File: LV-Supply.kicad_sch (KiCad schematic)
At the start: 20 parts, among them U11 LMR16006XDDCR

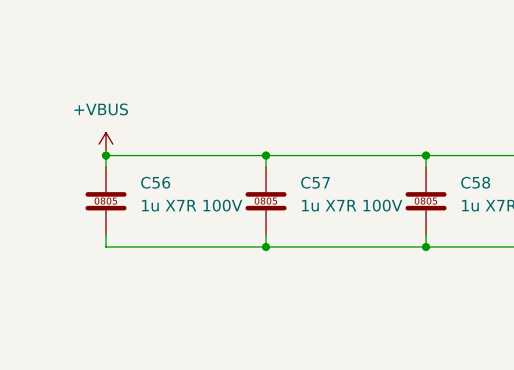
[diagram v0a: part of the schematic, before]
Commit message: Finished layout
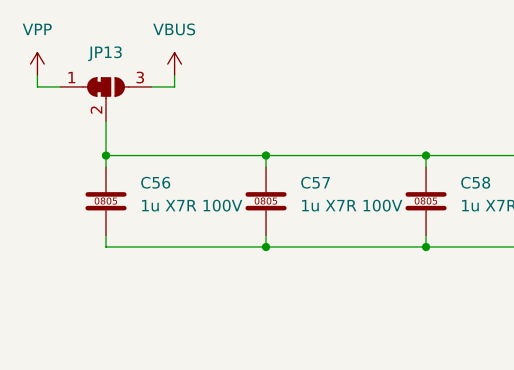
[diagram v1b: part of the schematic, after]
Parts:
- added JP13: SolderJumper_3_Bridged12, Jumper:SolderJumper-3_P1.3mm_Bridged12_RoundedPad1.0x1.5mm_NumberLabels, symbol Jumper:SolderJumper_3_Bridged12
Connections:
- net +VBUS: no longer names the net of C56.1, C57.1, C58.1, R81.1, U11.5 (IN)
- net +VBUS: now also JP13.2 (C)
- new net VBUS: JP13.3 (B)
- new net VPP: JP13.1 (A)
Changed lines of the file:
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@@
+	)
+	(junction
+		(at 39.37 74.93)
+		(diameter 0)
+		(color 0 0 0 0)
 	)
 	(junction
@@
 	)
 	(junction
-		(at 39.37 74.93)
-		(diameter 0)
-		(color 0 0 0 0)
-	)
-	(junction
 		(at 199.39 80.01)
 		(diameter 0)
@@
 	(wire
 		(pts
+			(xy 31.75 67.31) (xy 34.29 67.31)
+		)
+		(stroke
+			(width 0)
+			(type default)
+		)
+	)
+	(wire
+		(pts
 			(xy 100.33 74.93) (xy 124.46 74.93)
 		)
@@
 	(wire
 		(pts
+			(xy 39.37 71.12) (xy 39.37 74.93)
+		)
+		(stroke
+			(width 0)
+			(type default)
+		)
+	)
+	(wire
+		(pts
 			(xy 124.46 102.87) (xy 123.19 102.87)
 		)
@@
 	(wire
 		(pts
+			(xy 46.99 67.31) (xy 44.45 67.31)
+		)
+		(stroke
+			(width 0)
+			(type default)
+		)
+	)
+	(wire
+		(pts
 			(xy 199.39 110.49) (xy 199.39 113.03)
 		)
@@
 	(wire
 		(pts
+			(xy 46.99 66.04) (xy 46.99 67.31)
+		)
+		(stroke
+			(width 0)
+			(type default)
+		)
+	)
+	(wire
+		(pts
 			(xy 154.94 80.01) (xy 177.8 80.01)
 		)
@@
 		(pts
 			(xy 149.86 80.01) (xy 154.94 80.01)
+		)
+		(stroke
+			(width 0)
+			(type default)
+		)
+	)
+	(wire
+		(pts
+			(xy 31.75 66.04) (xy 31.75 67.31)
 		)
 		(stroke
@@
 	)
 	(symbol
+		(lib_id "power:VPP")
+		(at 31.75 66.04 0)
+		(unit 1)
+		(body_style 1)
+		(exclude_from_sim no)
+		(in_bom yes)
+		(on_board yes)
+		(in_pos_files yes)
+		(dnp no)
+		(fields_autoplaced yes)
+		(property "Reference" "#PWR021"
+			(at 31.75 69.85 0)
+			(hide yes)
+			(show_name no)
+			(do_not_autoplace no)
+			(effects
+				(font
+					(size 1.27 1.27)
+				)
+			)
+		)
+		(property "Value" "VPP"
+			(at 31.75 60.96 0)
+			(show_name no)
+			(do_not_autoplace no)
+			(effects
+				(font
+					(size 1.27 1.27)
+				)
+			)
+		)
+		(property "Footprint" ""
+			(at 31.75 66.04 0)
+			(hide yes)
+			(show_name no)
+			(do_not_autoplace no)
+			(effects
+				(font
+					(size 1.27 1.27)
+				)
+			)
+		)
+		(property "Datasheet" ""
+			(at 31.75 66.04 0)
+			(hide yes)
+			(show_name no)
+			(do_not_autoplace no)
+			(effects
+				(font
+					(size 1.27 1.27)
+				)
+			)
+		)
+		(property "Description" "Power symbol creates a global label with name \"VPP\""
+			(at 31.75 66.04 0)
+			(hide yes)
+			(show_name no)
+			(do_not_autoplace no)
+			(effects
+				(font
+					(size 1.27 1.27)
+				)
+			)
+		)
+		(pin "1"
+		)
+		(instances
+			(project "nitride-nano"
+				(path "/aaad0350-e7db-44d5-b7ef-99e6416f6948/7f7c4e65-0f35-4876-a2f6-d81218c9fb3e"
+					(reference "#PWR021")
+					(unit 1)
+				)
+			)
+		)
+	)
+	(symbol
 		(lib_id "power:+3V3")
 		(at 222.25 80.01 0)
@@
 	)
 	(symbol
+		(lib_id "power:VBUS")
+		(at 46.99 66.04 0)
+		(unit 1)
+		(body_style 1)
+		(exclude_from_sim no)
+		(in_bom yes)
+		(on_board yes)
+		(in_pos_files yes)
+		(dnp no)
+		(fields_autoplaced yes)
+		(property "Reference" "#PWR055"
+			(at 46.99 69.85 0)
+			(hide yes)
+			(show_name no)
+			(do_not_autoplace no)
+			(effects
+				(font
+					(size 1.27 1.27)
+				)
+			)
+		)
+		(property "Value" "VBUS"
+			(at 46.99 60.96 0)
+			(show_name no)
+			(do_not_autoplace no)
+			(effects
+				(font
+					(size 1.27 1.27)
+				)
+			)
+		)
+		(property "Footprint" ""
+			(at 46.99 66.04 0)
+			(hide yes)
+			(show_name no)
+			(do_not_autoplace no)
+			(effects
+				(font
+					(size 1.27 1.27)
+				)
+			)
+		)
+		(property "Datasheet" ""
+			(at 46.99 66.04 0)
+			(hide yes)
+			(show_name no)
+			(do_not_autoplace no)
+			(effects
+				(font
+					(size 1.27 1.27)
+				)
+			)
+		)
+		(property "Description" "Power symbol creates a global label with name \"VBUS\""
+			(at 46.99 66.04 0)
+			(hide yes)
+			(show_name no)
+			(do_not_autoplace no)
+			(effects
+				(font
+					(size 1.27 1.27)
+				)
+			)
+		)
+		(pin "1"
+		)
+		(instances
+			(project "nitride-nano"
+				(path "/aaad0350-e7db-44d5-b7ef-99e6416f6948/7f7c4e65-0f35-4876-a2f6-d81218c9fb3e"
+					(reference "#PWR055")
+					(unit 1)
+				)
+			)
+		)
+	)
+	(symbol
 		(lib_id "power:GND")
 		(at 199.39 113.03 0)
@@
 	)
 	(symbol
-		(lib_id "power:VBUS")
-		(at 39.37 74.93 0)
-		(unit 1)
-		(body_style 1)
-		(exclude_from_sim no)
-		(in_bom yes)
-		(on_board yes)
-		(in_pos_files yes)
-		(dnp no)
-		(property "Reference" "#PWR0156"
-			(at 39.37 74.93 0)
-			(hide yes)
-			(show_name no)
-			(do_not_autoplace no)
-			(effects
-				(font
-					(size 1.27 1.27)
-				)
-			)
-		)
-		(property "Value" "+VBUS"
-			(at 41.91 69.85 0)
-			(show_name no)
-			(do_not_autoplace no)
-			(effects
-				(font
-					(size 1.27 1.27)
-				)
-				(justify right)
-			)
-		)
-		(property "Footprint" ""
-			(at 39.37 74.93 0)
-			(show_name no)
-			(do_not_autoplace no)
-			(effects
-				(font
-					(size 1.27 1.27)
-				)
-			)
-		)
-		(property "Datasheet" ""
-			(at 39.37 74.93 0)
-			(show_name no)
-			(do_not_autoplace no)
-			(effects
-				(font
-					(size 1.27 1.27)
-				)
-			)
-		)
-		(property "Description" ""
-			(at 39.37 74.93 0)
-			(show_name no)
-			(do_not_autoplace no)
-			(effects
-				(font
-					(size 1.27 1.27)
-				)
-			)
-		)
-		(pin "1"
-		)
-		(instances
-			(project "nitride-nano"
-				(path "/aaad0350-e7db-44d5-b7ef-99e6416f6948/7f7c4e65-0f35-4876-a2f6-d81218c9fb3e"
-					(reference "#PWR0156")
-					(unit 1)
-				)
-			)
-		)
-	)
-	(symbol
 		(lib_id "0_passives:C_0805")
 		(at 39.37 80.01 0)
@@
 					(unit 1)
 				)
+			)
+		)
+	)
+	(symbol
+		(lib_id "Jumper:SolderJumper_3_Bridged12")
+		(at 39.37 67.31 0)
+		(unit 1)
+		(body_style 1)
+		(exclude_from_sim no)
+		(in_bom no)
+		(on_board yes)
+		(in_pos_files yes)
+		(dnp no)
+		(property "Reference" "JP13"
+			(at 39.37 63.5 0)
+			(show_name no)
+			(do_not_autoplace no)
+			(effects
+				(font
+					(size 1.27 1.27)
+				)
+			)
+		)
+		(property "Value" "SolderJumper_3_Bridged12"
+			(at 39.37 60.96 0)
+			(hide yes)
+			(show_name no)
+			(do_not_autoplace no)
+			(effects
+				(font
+					(size 1.27 1.27)
+				)
+			)
+		)
+		(property "Footprint" "Jumper:SolderJumper-3_P1.3mm_Bridged12_RoundedPad1.0x1.5mm_NumberLabels"
+			(at 39.37 67.31 0)
+			(hide yes)
+			(show_name no)
+			(do_not_autoplace no)
+			(effects
+				(font
+					(size 1.27 1.27)
+				)
+			)
+		)
+		(property "Datasheet" ""
+			(at 39.37 82.55 0)
+			(hide yes)
+			(show_name no)
+			(do_not_autoplace no)
+			(effects
+				(font
+					(size 1.27 1.27)
+				)
+			)
+		)
+		(property "Description" "3-pole Solder Jumper, pins 1+2 closed/bridged"
+			(at 39.37 80.01 0)
+			(hide yes)
+			(show_name no)
+			(do_not_autoplace no)
+			(effects
+				(font
+					(size 1.27 1.27)
+				)
+			)
+		)
+		(pin "3"
+		)
+		(pin "1"
+		)
+		(pin "2"
+		)
+		(instances
+			(project "nitride-nano"
+				(path "/aaad0350-e7db-44d5-b7ef-99e6416f6948/7f7c4e65-0f35-4876-a2f6-d81218c9fb3e"
+					(reference "JP13")
+					(unit 1)
+				)
